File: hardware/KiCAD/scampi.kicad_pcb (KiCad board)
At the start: 2 copper layers, 20 x 20 mm, 58 parts, among them IC1 LSF0204GU12X, J1 AudioJack3_SwitchT, U1 MIC5365-1.8YC5-TR, U2 TLV320AIC3100, U3 ATTINY1616-MNR

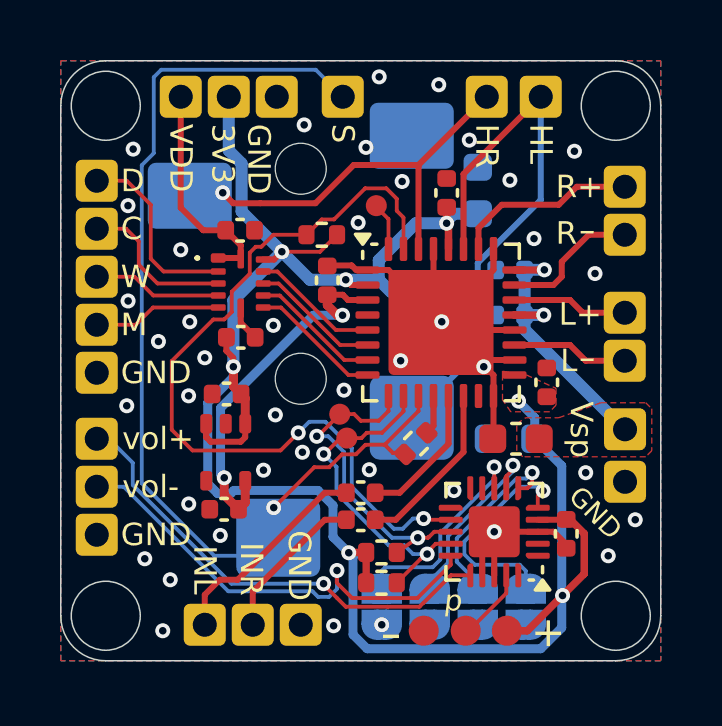
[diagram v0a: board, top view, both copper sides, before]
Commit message: board tweaks & firmware
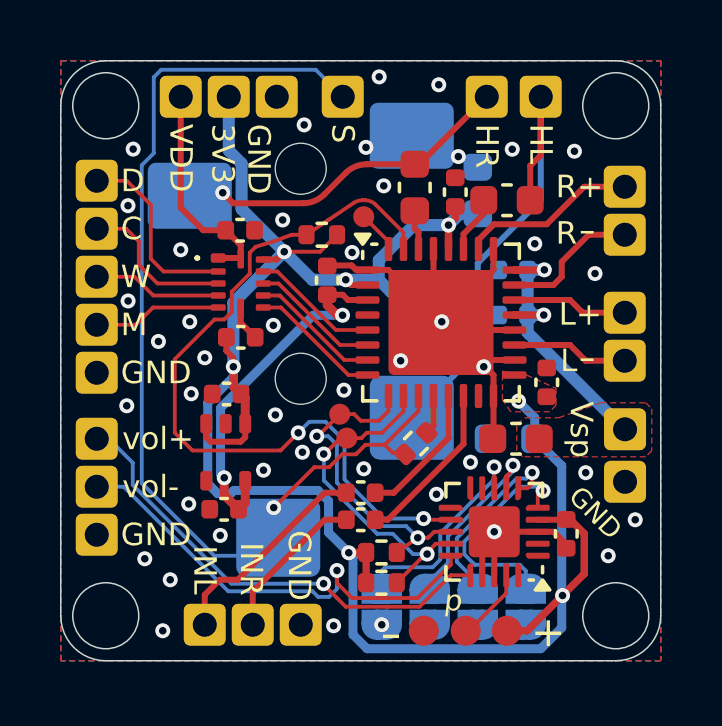
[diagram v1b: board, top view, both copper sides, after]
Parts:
- added C17: 47µF, Capacitor_SMD:C_0603_1608Metric, F.Cu at (152.9, 89.7)
- added C18: 47µF, Capacitor_SMD:C_0603_1608Metric, F.Cu at (149.8, 89.2)
- C13, C14: value 0.47µF -> 1µF
- moved TP7 0.56 mm to (148.1, 90.2)
- moved C9 0.29 mm to (151.2, 89.4)
- moved C11 0.10 mm to (153.1, 92.0)
- moved C12 0.10 mm to (153.1, 93.5)
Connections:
- U2 pad 27: /HPL -> Net-(U2-HPL)
- U2 pad 30: /HPR -> Net-(U2-HPR)
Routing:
- net /HPR: track 13.2 -> 10.3 mm
- net /HPL: track 18.6 -> 16.1 mm
- net Net-(U2-HPL): track 0.00 -> 1.90 mm
- net RES: track 27.3 -> 25.8 mm
- net Net-(U2-HPR): track 0.00 -> 1.33 mm
- net GND: vias 41 -> 43
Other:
- outline, holes or cut-outs redrawn
- board text added: "<"

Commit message: firmware, new layout
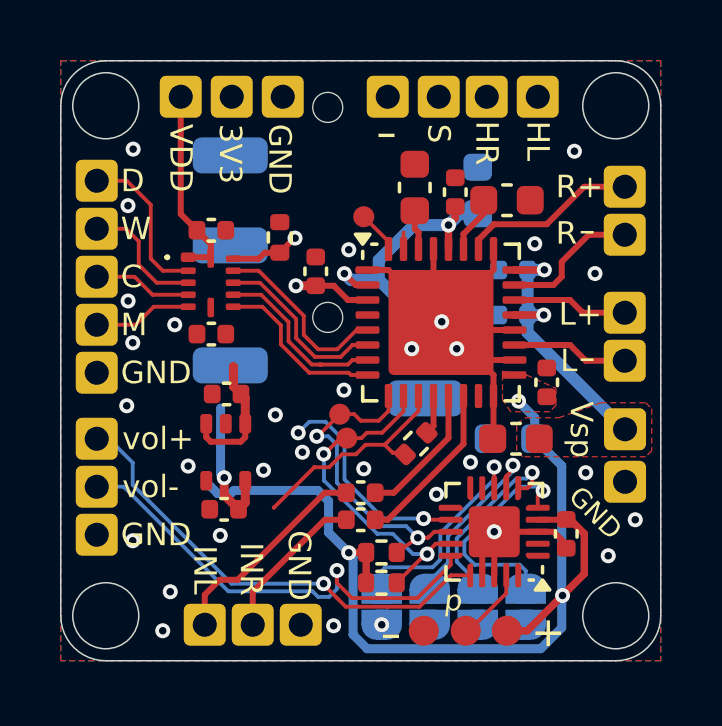
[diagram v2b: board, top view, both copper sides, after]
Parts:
- removed DET1, HPL1, HPR1: ~, SamacSys_Parts:pth_pad
- removed J1: AudioJack3_SwitchT, Connector_Audio:Jack_3.5mm_CUI_SJ-3524-SMT_Horizontal
- added ?: , , F.Cu at (150.6, 86.2)
- added ?: , , F.Cu at (153.9, 86.2)
- added ?: , , F.Cu at (152.2, 86.2)
- added ?: , , F.Cu at (148.9, 86.2)
- added J2: PJ-320D, SamacSys_Parts:Jack_3.5mm_PJ320D_Horizontal, B.Cu at (146.9, 91.3)
- moved TP7 1.60 mm to (139.2, 92.2)
- moved TP8 1.60 mm to (139.2, 90.6)
- moved R1 1.40 mm to (145.3, 90.9), turned to -90 degrees
- moved C10 1.10 mm to (151.3, 92.7)
- moved IC1 1.00 mm to (143.0, 92.4)
- moved C3 0.99 mm to (143.0, 94.1), turned to 180 degrees
- moved C2 0.96 mm to (143.0, 90.6)
- moved C5 0.49 mm to (146.5, 92.0)
- moved TP3 0.20 mm to (145.4, 86.2)
- moved TP4 0.10 mm to (143.7, 86.2)
- renumbered C16 to C13, C17 to C14, C18 to C15, C13 to C16, C14 to C17, C15 to C18, R4 to R1, R1 to R2, R2 to R3, R3 to R4, TP15 to TP1, TP6 to TP10, TP7 to TP11, TP8 to TP12, TP9 to TP13, TP10 to TP14, TP11 to TP15, TP12 to TP16, TP13 to TP17, TP14 to TP18, TP16 to TP2, TP17 to TP3, TP18 to TP4, TP1 to TP5, TP2 to TP6, TP3 to TP7, TP4 to TP8, TP5 to TP9
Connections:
- IC1 pad 3: /C_IN -> /W_IN
- IC1 pad 4: /W_IN -> /C_IN
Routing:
- net /HPS: track 33.7 -> 7.47 mm, vias 1 -> 0
- net RES: track 25.8 -> 7.89 mm
- net +3V3: track 67.5 -> 50.1 mm, vias 7 -> 6
- net /HPL: track 16.1 -> 0.34 mm
- net /HPR: track 10.3 -> 0.00 mm, vias 1 -> 0
- net +1V8: track 12.4 -> 7.15 mm
- net GND: track 27.5 -> 25.2 mm, vias 43 -> 31
- net /D: track 4.28 -> 6.48 mm
- net /C_IN: track 5.26 -> 3.30 mm
- net /W: track 4.32 -> 6.04 mm
- net /C: track 4.37 -> 5.98 mm
- net /M: track 4.41 -> 5.79 mm
- net /D_IN: track 6.36 -> 5.35 mm
- net /M_IN: track 4.29 -> 3.30 mm
- net VDDIO_EXT: track 7.43 -> 6.55 mm
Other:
- board text added: "HPS"
- board text removed: "<"

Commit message: layout changes, ADC test fw
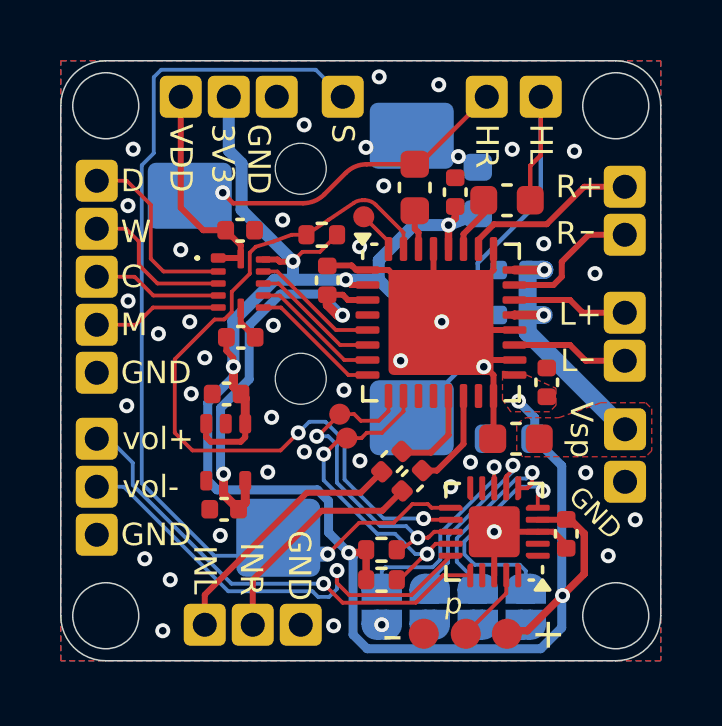
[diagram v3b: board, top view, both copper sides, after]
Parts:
- removed ? (x4): , 
- removed J2: PJ-320D, SamacSys_Parts:Jack_3.5mm_PJ320D_Horizontal
- removed the R2 at (149.8, 97.8)
- added DET1: ~, SamacSys_Parts:pth_pad, F.Cu at (147.4, 86.2)
- added HPL1: ~, SamacSys_Parts:pth_pad, F.Cu at (154.0, 86.2)
- added HPR1: ~, SamacSys_Parts:pth_pad, F.Cu at (152.2, 86.2)
- added J1: AudioJack3_SwitchT, Connector_Audio:Jack_3.5mm_CUI_SJ-3524-SMT_Horizontal, B.Cu at (146.0, 91.1)
- moved C14 2.16 mm to (149.7, 99.0), turned to -135 degrees
- moved C13 1.47 mm to (149.0, 98.4), turned to -135 degrees
- moved R4 1.40 mm to (146.7, 90.8), turned to 0 degrees
- moved C10 1.10 mm to (150.2, 92.7)
- moved IC1 1.00 mm to (144.0, 92.4)
- moved C3 0.99 mm to (144.0, 94.2), turned to 0 degrees
- moved C2 0.96 mm to (144.0, 90.6)
- moved C5 0.49 mm to (146.9, 92.3)
- moved TP17 0.20 mm to (145.2, 86.2)
- moved R2 0.10 mm to (148.7, 102.3)
- moved TP12 0.10 mm to (152.9, 104.1)
- moved TP14 0.10 mm to (150.1, 104.1)
- moved TP18 0.10 mm to (143.6, 86.2)
- moved UPDI1 0.10 mm to (151.5, 104.1)
- moved R3 0.09 mm to (148.7, 101.3)
- renumbered C16 to C13, C17 to C14, C18 to C15, C13 to C16, C14 to C17, C15 to C18, R3 to R2, R4 to R3, R1 to R4, TP5 to TP1, TP14 to TP10, TP15 to TP11, TP16 to TP12, TP17 to TP13, TP18 to TP14, TP1 to TP15, TP2 to TP16, TP3 to TP17, TP4 to TP18, TP6 to TP2, TP7 to TP3, TP8 to TP4, TP9 to TP5, TP10 to TP6, TP11 to TP7, TP12 to TP8, TP13 to TP9
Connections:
- U2 pad 11: /HPS -> unconnected-(U2-VOL/MICDET-Pad11)
- U2 pad 12: Net-(U2-MICBIAS) -> unconnected-(U2-MICBIAS-Pad12)
- U3 pad 11: GND -> /HPS
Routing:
- net /HPS: track 7.47 -> 35.6 mm, vias 0 -> 1
- net RES: track 7.89 -> 25.8 mm
- net +3V3: track 50.1 -> 67.2 mm, vias 6 -> 7
- net /HPL: track 0.34 -> 16.1 mm
- net /HPR: track 0.00 -> 10.3 mm, vias 0 -> 1
- net +1V8: track 7.15 -> 14.1 mm
- net Net-(C14-Pad2): track 5.21 -> 7.71 mm
- net Net-(U2-MIC1RP): track 5.59 -> 3.33 mm
- net /D: track 6.48 -> 4.28 mm
- net /W: track 6.04 -> 4.32 mm
- net /C: track 5.98 -> 4.37 mm
- net Net-(U2-MIC1LP): track 4.60 -> 3.05 mm
- net Net-(C13-Pad2): track 7.13 -> 8.60 mm
- net /M: track 5.79 -> 4.41 mm
- net Net-(U2-MICBIAS): track 1.32 -> 0.00 mm
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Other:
- board text added: "<"
- board text removed: "HPS"
